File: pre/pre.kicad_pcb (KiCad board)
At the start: 2 copper layers, 19.8 x 84.3 mm, 35 parts, among them J5 Conn_02x05_Odd_Even, U1 TL072, U2 TL072

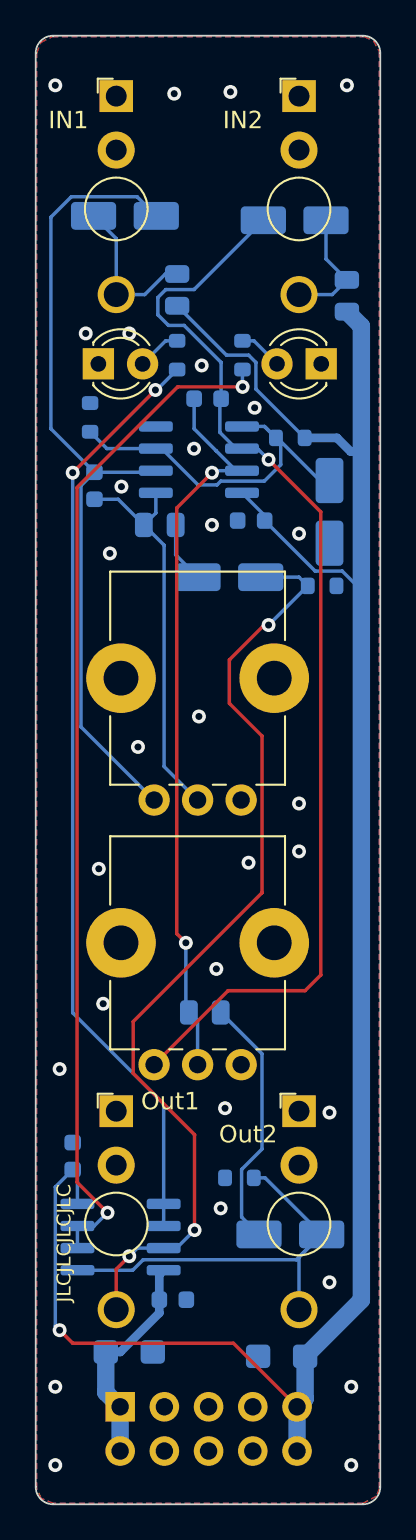
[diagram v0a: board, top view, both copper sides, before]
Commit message: Alignment Fix
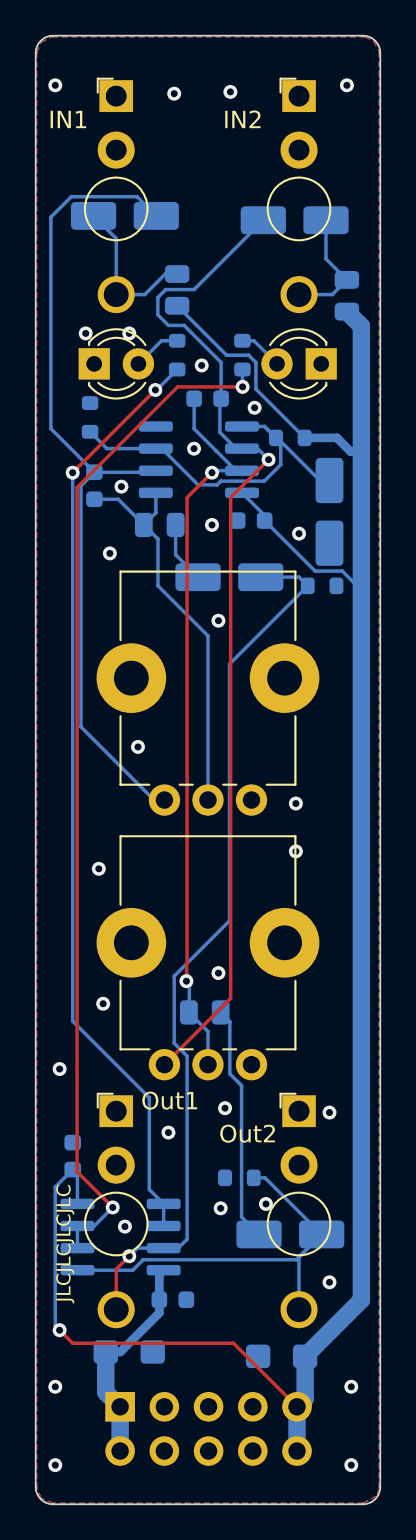
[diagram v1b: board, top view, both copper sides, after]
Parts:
- moved RV1 0.60 mm to (90.8, 98.8)
- moved RV2 0.60 mm to (90.8, 114.0)
- moved LED1 0.24 mm to (81.7, 73.8)
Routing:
- net pot_a_R: track 63.7 -> 58.4 mm
- net Net-(C1-Pad2): track 55.1 -> 51.2 mm, vias 3 -> 1
- net Net-(C4-Pad1): track 14.6 -> 13.7 mm
- net pot_a_L: track 47.1 -> 47.7 mm
- net GND: vias 30 -> 32
